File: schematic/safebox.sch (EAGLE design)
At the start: 15 parts, among them U1 M-04522_FXMA108

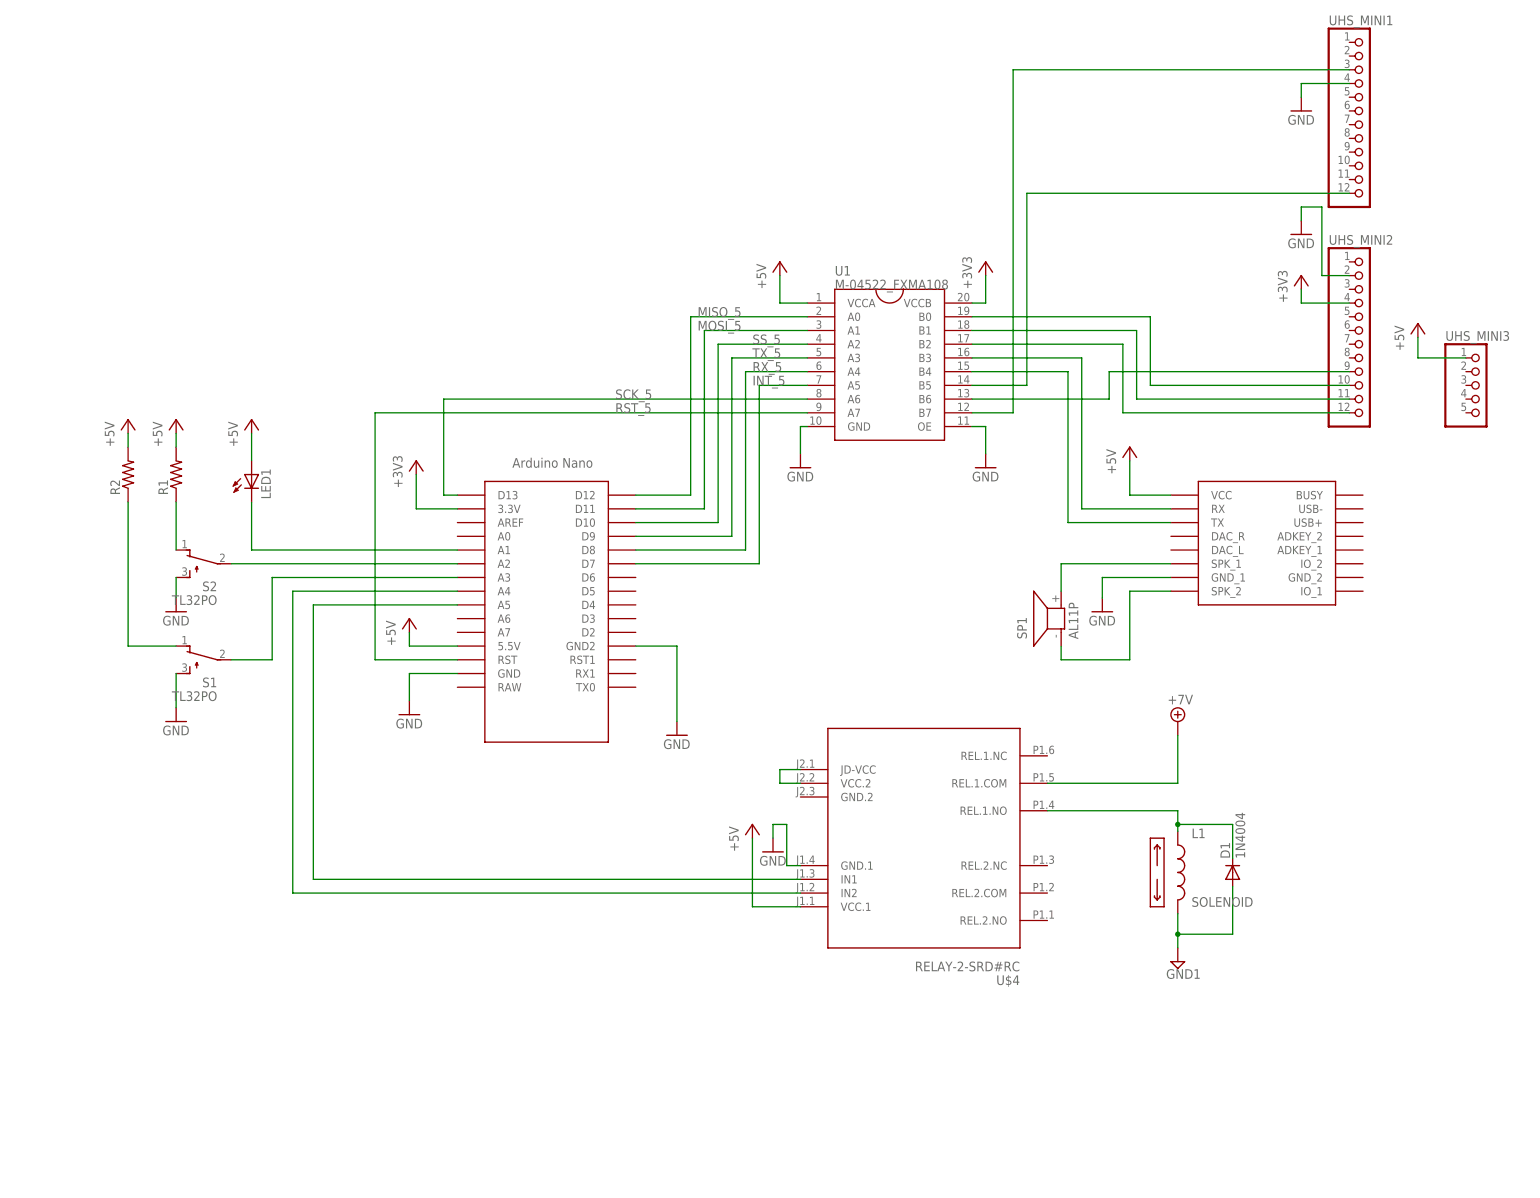
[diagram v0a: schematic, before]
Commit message: 回路図修正
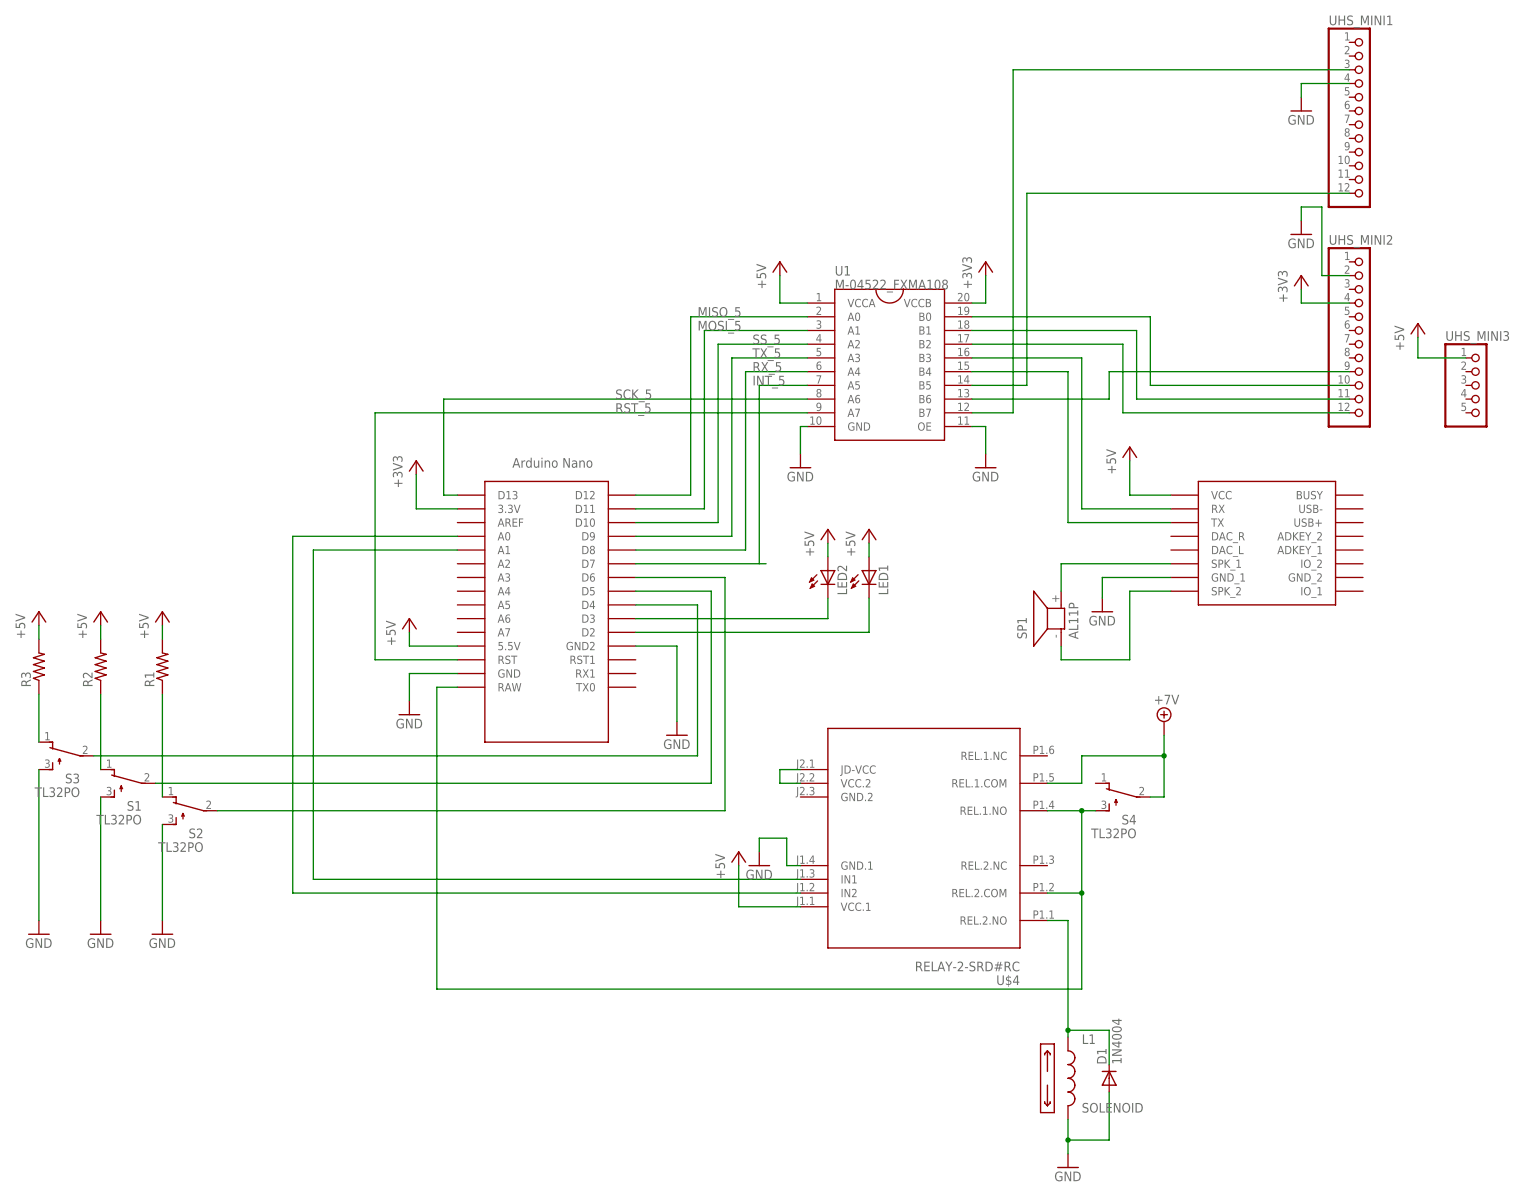
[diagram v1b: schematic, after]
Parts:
- added LED2: (no value), led:LED10MM
- added R3: (no value), resistor:R-US_0207/12
- added S3, S4: TL32PO, switch:TL32PO
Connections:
- removed net GND1: D1.A, L1.2
- new net N$15: R3.1, S3.O
- new net N$16: S3.P, U$1.D4
- new net N$22: S2.P, U$1.D6
- new net N$23: U$1.D7
- new net N$24: S4.S, U$1.RAW, U$4.REL.1.NO, U$4.REL.2.COM
- net +5V: now also LED2.A, R3.2
- net +7V: now also S4.P
- net GND: now also D1.A, L1.2, S3.S
- net INT_5: no longer U$1.D7
- net N$12: now also U$1.A0; no longer U$1.A4
- net N$13: now also U$1.A1; no longer U$1.A5
- net N$14: now also U$4.REL.2.NO; no longer U$4.REL.1.NO
- net N$19: now also U$1.D5; no longer U$1.A3
- net N$20: now also LED2.C, U$1.D3; no longer S2.P, U$1.A2
- net N$21: now also U$1.D2; no longer U$1.A1
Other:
- moved on the sheet: D1, L1, LED1, R1, R2, S1, S2
